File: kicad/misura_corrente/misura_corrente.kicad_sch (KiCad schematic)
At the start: 16 parts, among them U0 CA3140, U1 CA3140, U3 INA111

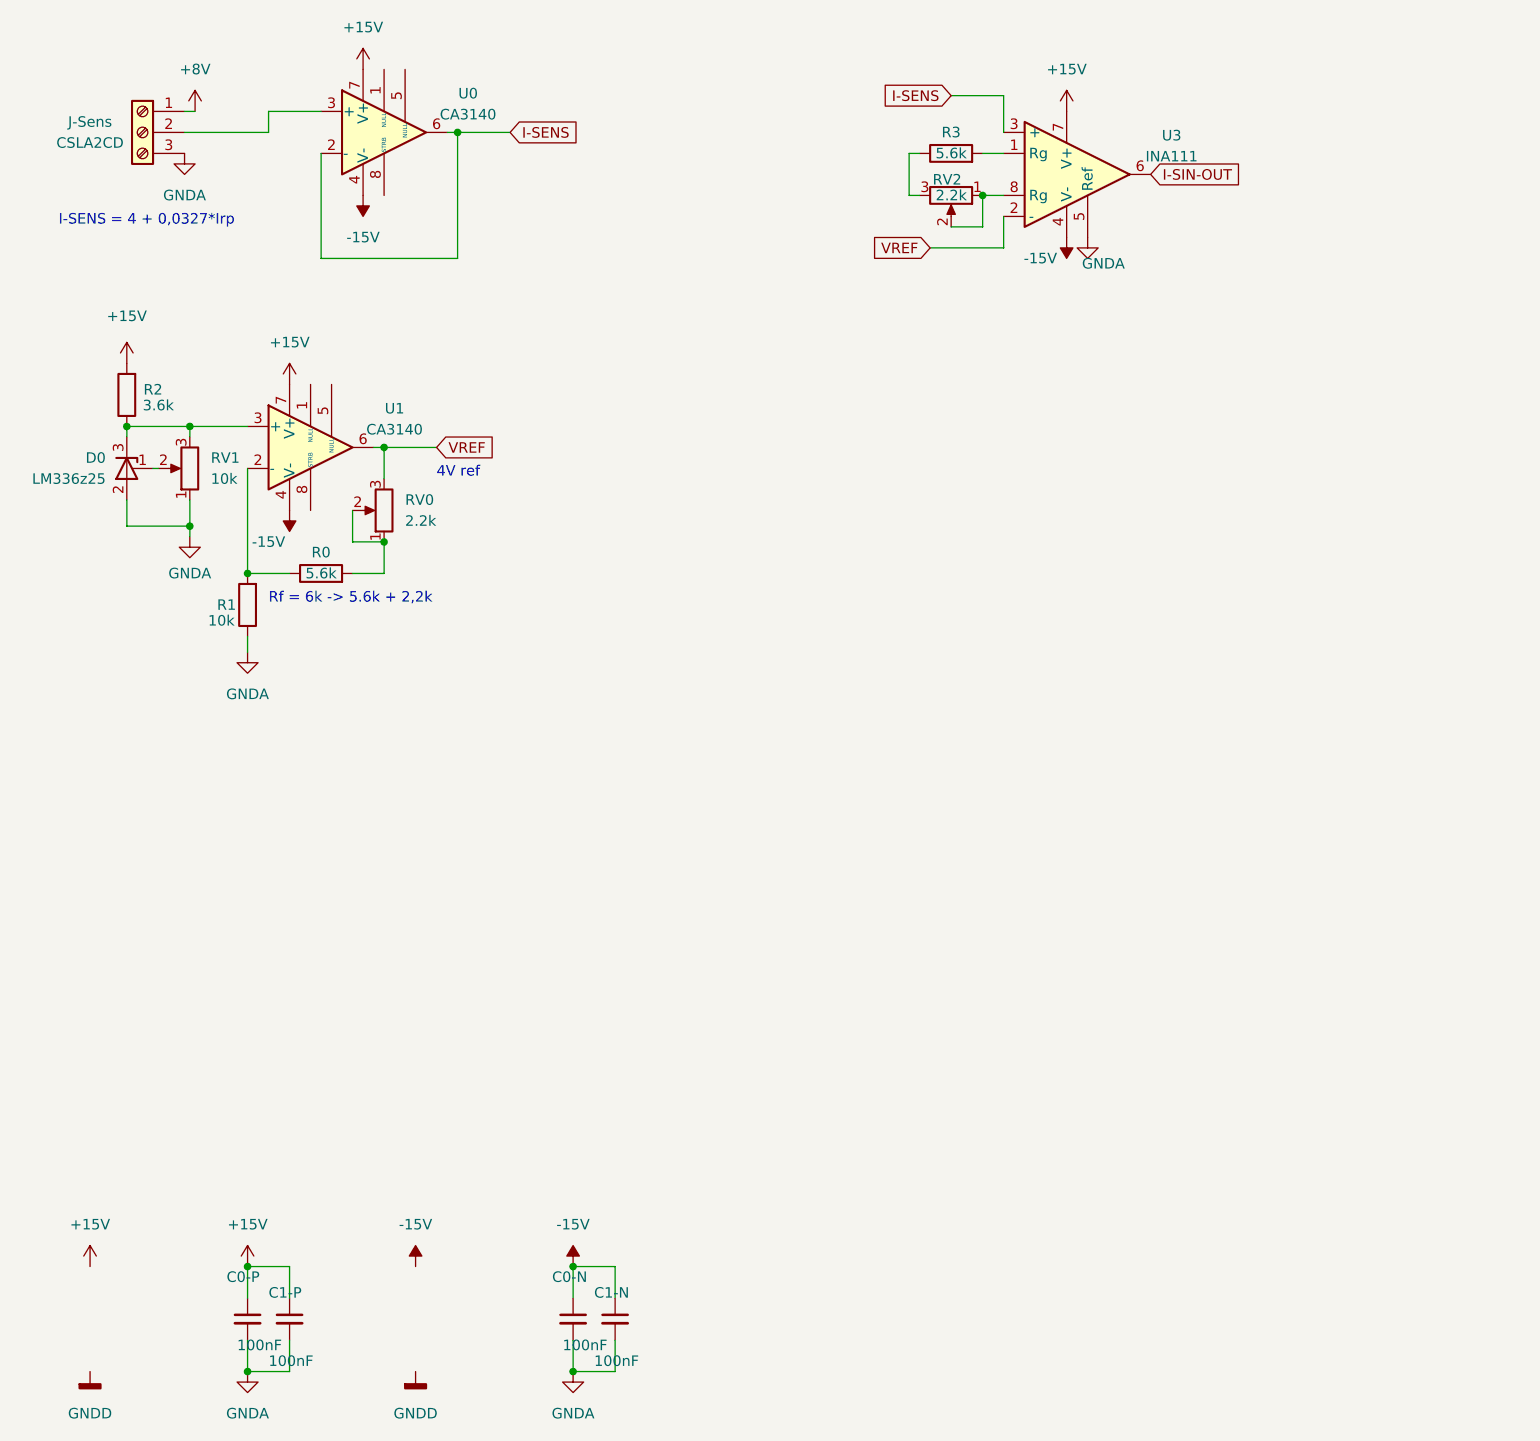
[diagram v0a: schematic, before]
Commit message: boh
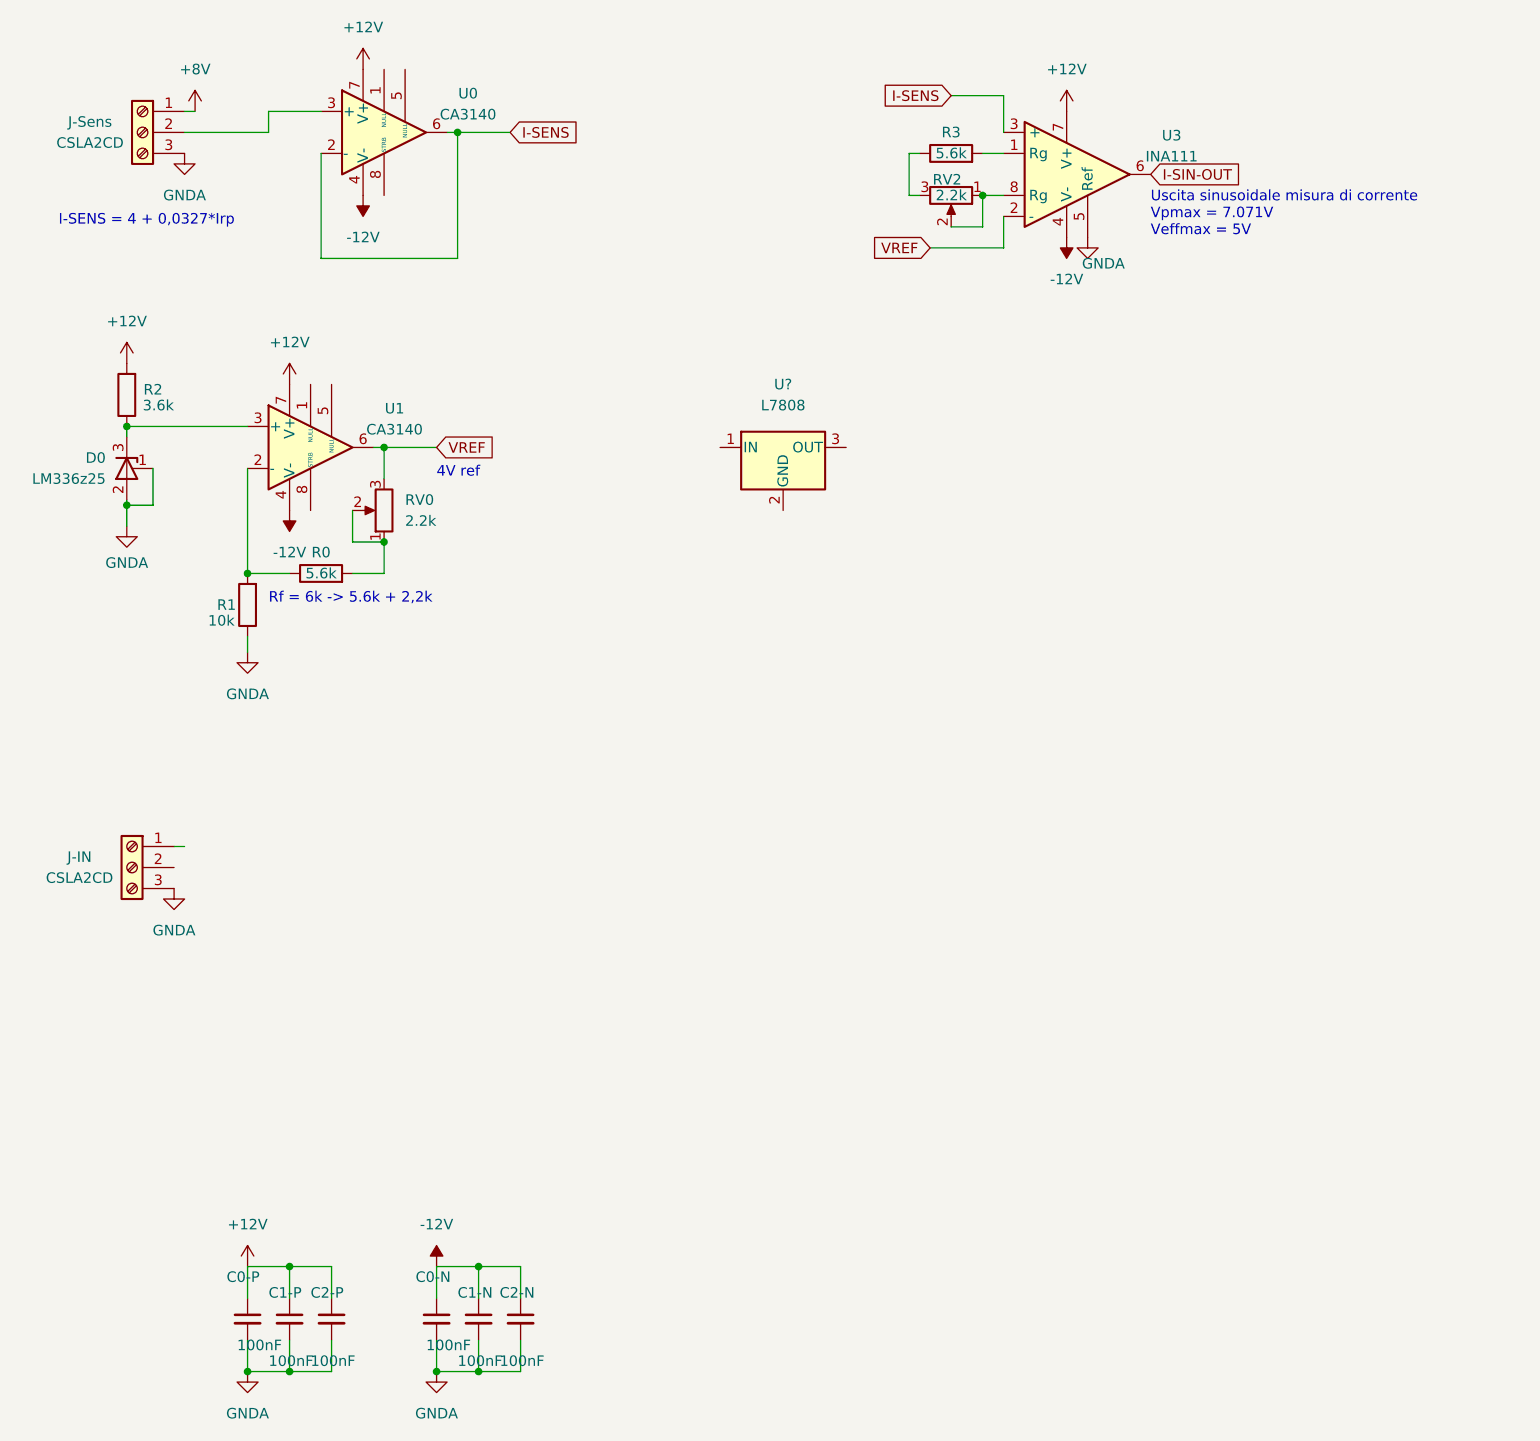
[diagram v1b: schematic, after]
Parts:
- removed RV1: 10k, symbol Device:R_Potentiometer
- added C2-N, C2-P: 100nF, symbol Device:C_Small
- added J-IN: CSLA2CD, symbol Connector:Screw_Terminal_01x03
- added U?: L7808, symbol Regulator_Linear:L7808
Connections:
- net GNDA: now also D0.1 (Adj), C2-N.2, C2-P.2, J-IN.3 (Pin_3)
- net +15V renamed +12V
- net +12V: now also C2-P.1
- net -15V renamed -12V
- net -12V: now also C2-N.1
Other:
- note added: "Uscita sinusoidale misura di corrente Vpmax = 7.071V Veffmax = 5V"
- moved on the sheet: C0-N, C1-N
